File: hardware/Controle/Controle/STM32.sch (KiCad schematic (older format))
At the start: 18 parts, among them U501 STM32F103C8Tx, Y501 8mhz

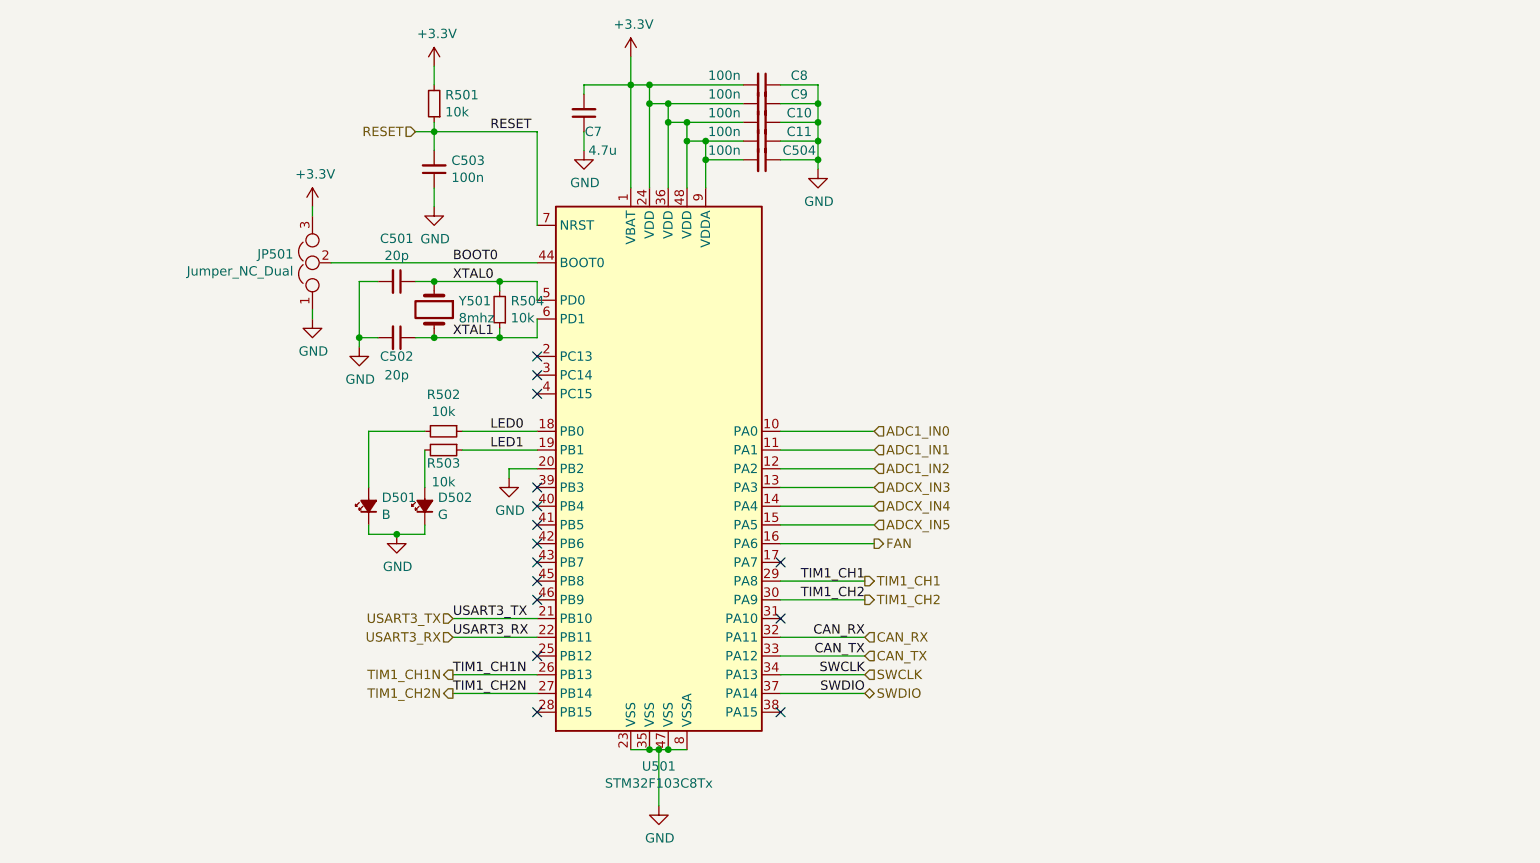
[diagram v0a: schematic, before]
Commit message: Update Controle PCB
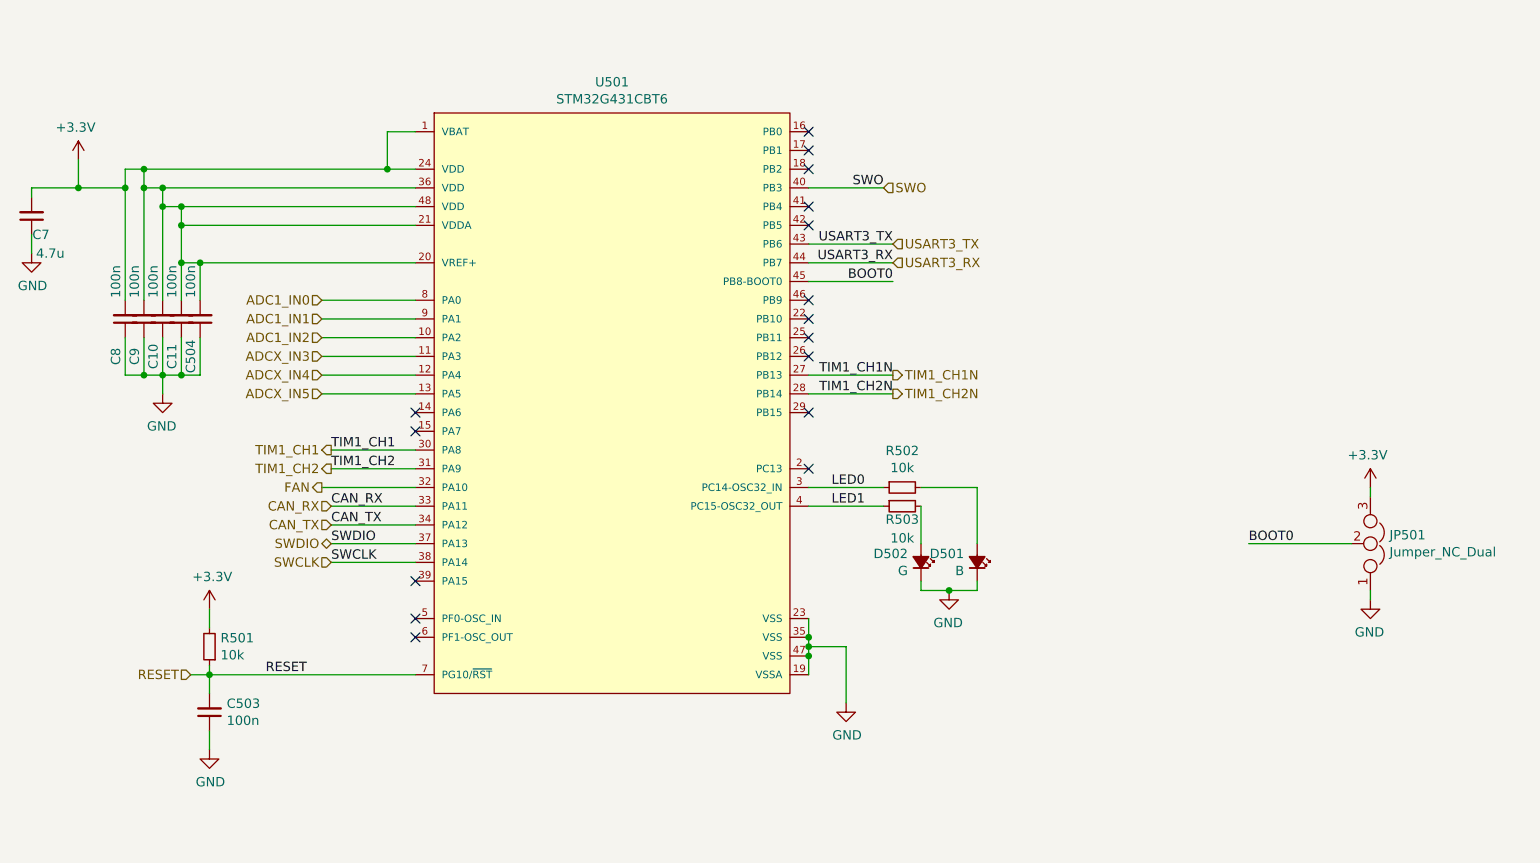
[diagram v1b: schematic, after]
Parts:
- removed C501, C502: 20p, Capacitor_SMD:C_0603_1608Metric_Pad1.08x0.95mm_HandSolder, symbol Device:C_Small
- removed R504: 10k, Resistor_SMD:R_0603_1608Metric_Pad0.98x0.95mm_HandSolder, symbol Device:R_Small
- removed U501: STM32F103C8Tx, Package_QFP:LQFP-48_7x7mm_P0.5mm, symbol MCU_ST_STM32F1:STM32F103C8Tx
- removed Y501: 8mhz, Crystal:Crystal_SMD_HC49-SD, symbol Device:Crystal
- added U501: STM32G431CBT6, Package_QFP:LQFP-48_7x7mm_P0.5mm, symbol STM32G431C8T6:STM32G431CBT6
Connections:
- net +3V3: now also U501.1 (VBAT), U501.20 (VREF+), U501.21 (VDDA), U501.24 (VDD), U501.36 (VDD), U501.48 (VDD)
- net ADC1_IN0: now also U501.8 (PA0)
- net ADC1_IN1: now also U501.9 (PA1)
- net ADC1_IN2: now also U501.10 (PA2)
- net ADCX_IN3: now also U501.11 (PA3)
- net ADCX_IN4: now also U501.12 (PA4)
- net ADCX_IN5: now also U501.13 (PA5)
- net BOOT0: now also U501.45 (PB8-BOOT0)
- net CAN_RX: now also U501.33 (PA11)
- net CAN_TX: now also U501.34 (PA12)
- net FAN: now also U501.32 (PA10)
- net GND: now also U501.19 (VSSA), U501.23 (VSS), U501.35 (VSS), U501.47 (VSS)
- net LED0: now also U501.3 (PC14-OSC32_IN)
- net LED1: now also U501.4 (PC15-OSC32_OUT)
- net RESET: now also U501.7 (PG10/~RST~)
- net SWCLK: now also U501.38 (PA14)
- net SWDIO: now also U501.37 (PA13)
- net TIM1_CH1: now also U501.30 (PA8)
- net TIM1_CH1N: now also U501.27 (PB13)
- net TIM1_CH2: now also U501.31 (PA9)
- net TIM1_CH2N: now also U501.28 (PB14)
- net USART3_RX: now also U501.44 (PB7)
- net USART3_TX: now also U501.43 (PB6)
- new net SWO: U501.40 (PB3)
- no-connect marks 15 -> 16
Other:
- moved on the sheet: C10, C11, C503, C504, C7, C8, C9, D501, D502, JP501, R501, R502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
